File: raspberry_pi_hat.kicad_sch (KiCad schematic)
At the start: 30 parts, among them J1 CONN_JTAG, J3 Conn_01x08, J4 475890001, P1 CONN_02X20, U1 93LC56BT-I_OT, U2 FT232H, Y1 CSTNE12M0G550000R0

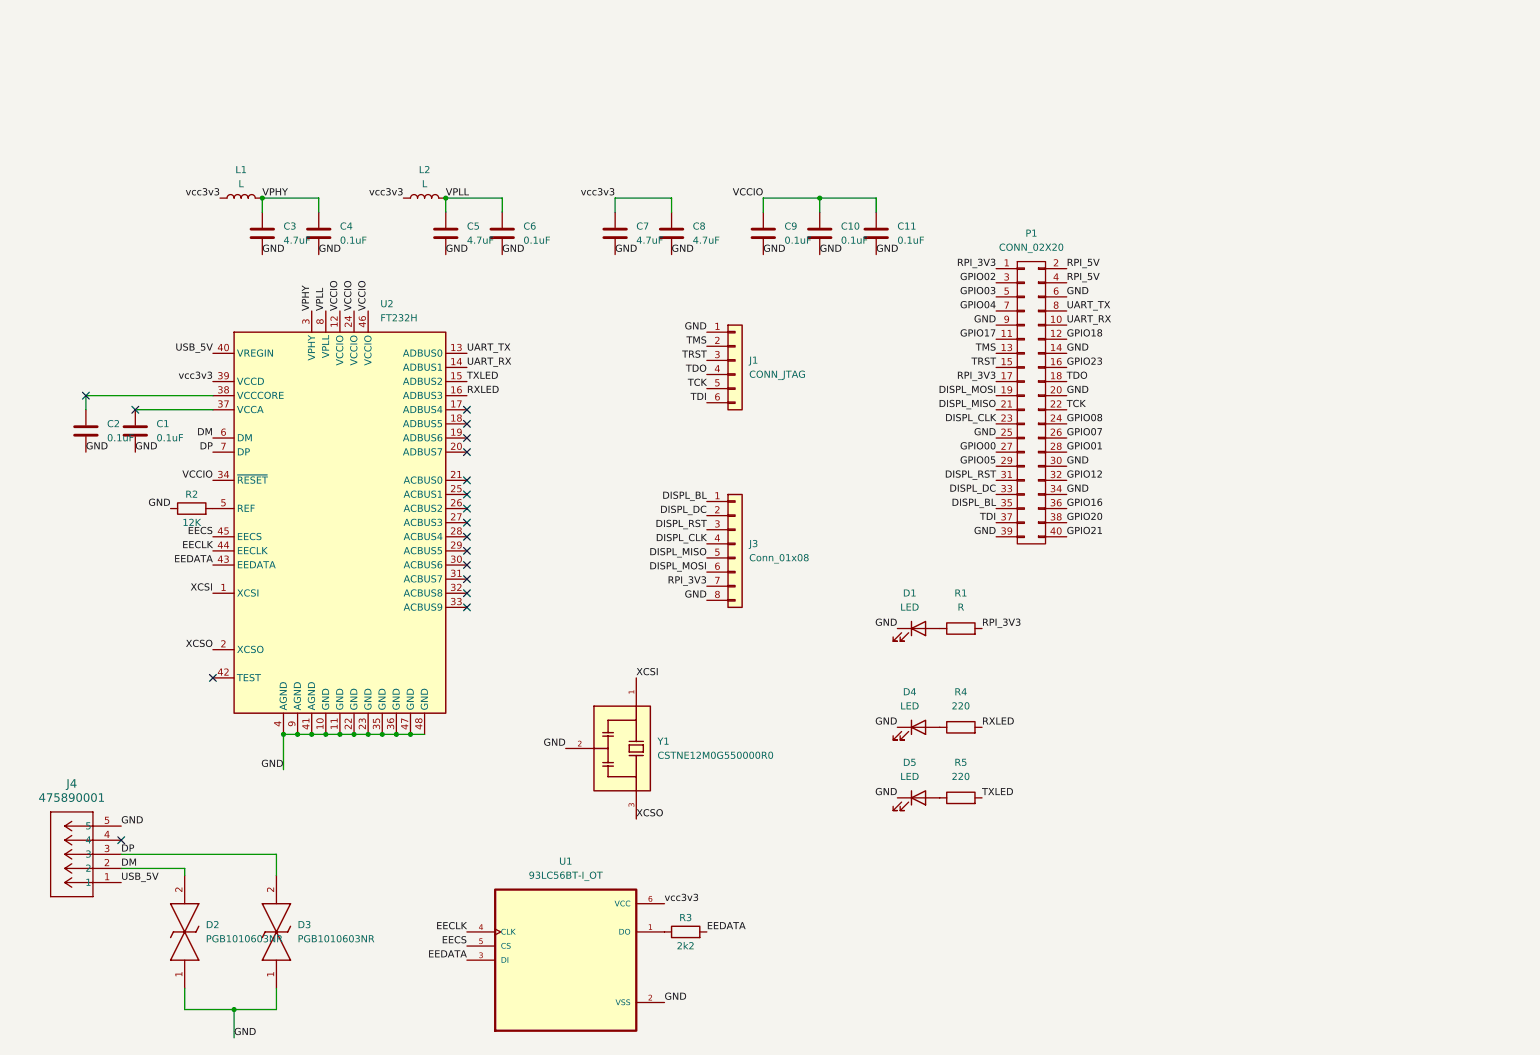
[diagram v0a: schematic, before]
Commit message: progress
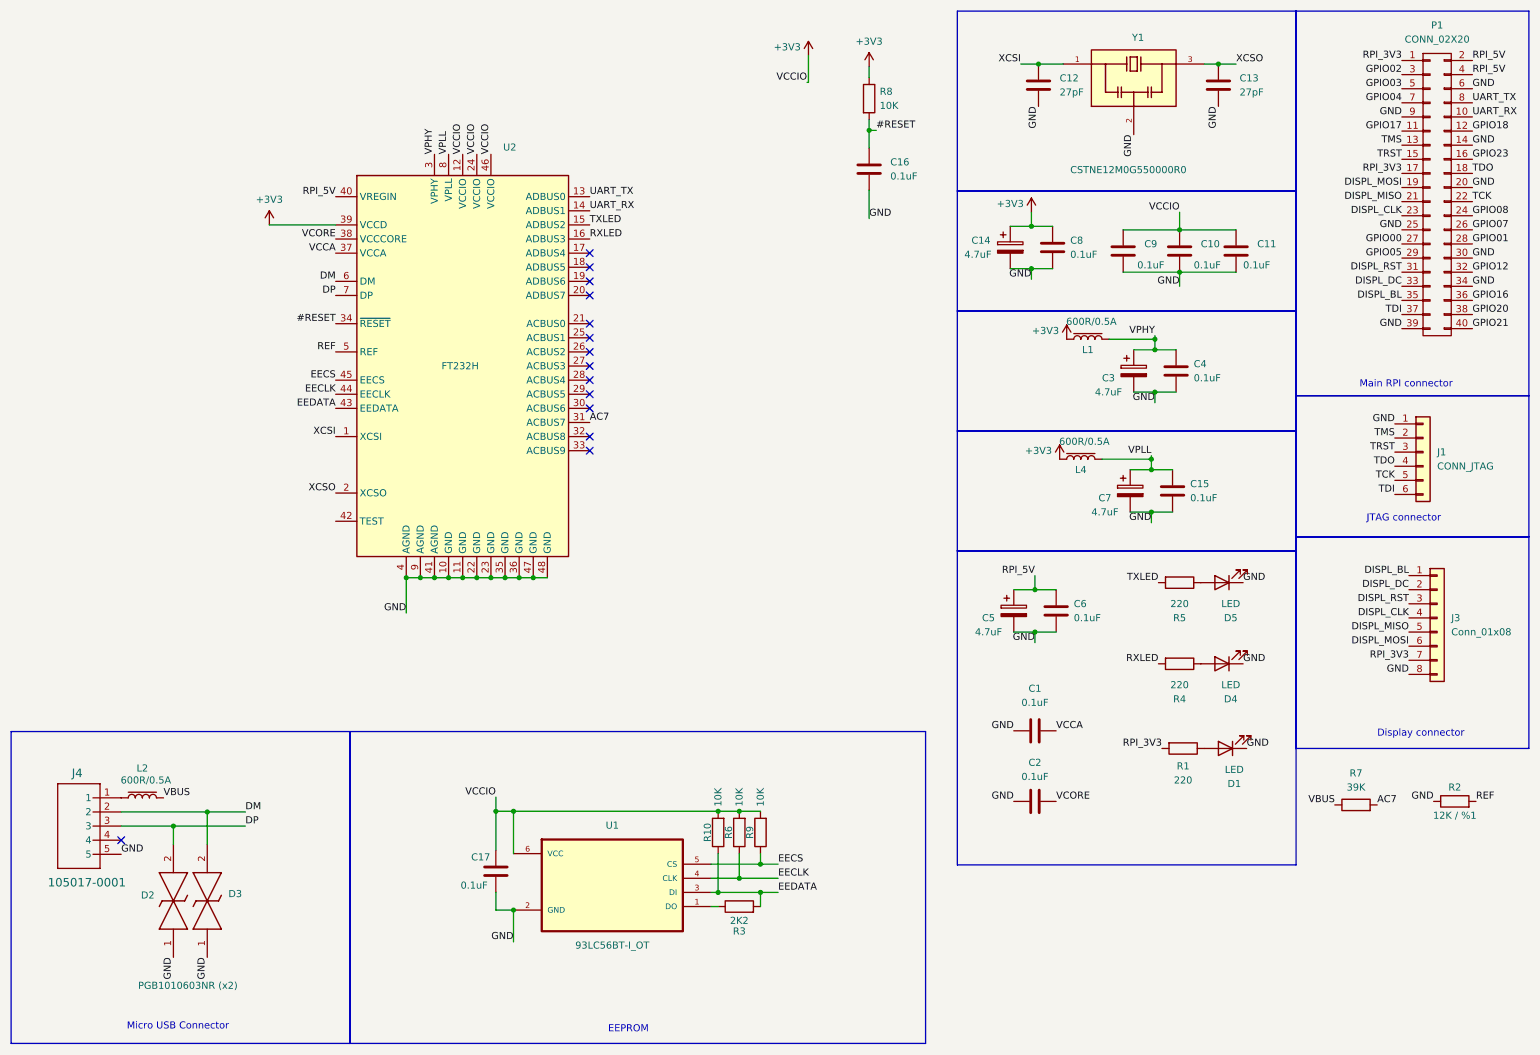
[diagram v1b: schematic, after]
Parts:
- removed C3, C5, C7: 4.7uF, Capacitor_SMD:C_0504_1310Metric_Pad0.83x1.28mm_HandSolder, symbol Device:C
- removed L1, L2: L, Inductor_SMD:L_1008_2520Metric, symbol Device:L
- added C12, C13: 27pF, Capacitor_SMD:C_0201_0603Metric_Pad0.64x0.40mm_HandSolder, symbol Device:C
- added C14, C3, C5, C7: 4.7uF, footprints:CAPPM2014X120N, symbol Device:C_Polarized
- added C15, C16, C17: 0.1uF, Capacitor_SMD:C_0201_0603Metric_Pad0.64x0.40mm_HandSolder, symbol Device:C
- added L1, L2, L4: 600R/0.5A, footprints:BLM21AG102BH1J, symbol Device:L_Iron
- added R10, R6, R8, R9: 10K, Resistor_SMD:R_0201_0603Metric_Pad0.64x0.40mm_HandSolder, symbol Device:R
- added R7: 39K, Resistor_SMD:R_0201_0603Metric_Pad0.64x0.40mm_HandSolder, symbol Device:R
- C1, C10, C11, C2, C4, C6, C9: footprint Capacitor_SMD:C_0504_1310Metric_Pad0.83x1.28mm_HandSolder -> Capacitor_SMD:C_0201_0603Metric_Pad0.64x0.40mm_HandSolder
- C8: value 4.7uF -> 0.1uF; footprint Capacitor_SMD:C_0504_1310Metric_Pad0.83x1.28mm_HandSolder -> Capacitor_SMD:C_0201_0603Metric_Pad0.64x0.40mm_HandSolder
- D2: value PGB1010603NR -> PGB1010603NR (x2)
- J4: value 475890001 -> 105017-0001; Product (none) -> https://www.mouser.fr/ProductDetail/Molex/105017-0001?qs=hl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
- R1: value R -> 220; footprint Resistor_SMD:R_0603_1608Metric -> Resistor_SMD:R_0201_0603Metric_Pad0.64x0.40mm_HandSolder
- R2: value 12K -> 12K / %1; footprint Resistor_SMD:R_0402_1005Metric_Pad0.72x0.64mm_HandSolder -> Resistor_SMD:R_0201_0603Metric_Pad0.64x0.40mm_HandSolder
- R3: value 2k2 -> 2K2; footprint Resistor_SMD:R_0402_1005Metric_Pad0.72x0.64mm_HandSolder -> Resistor_SMD:R_0201_0603Metric_Pad0.64x0.40mm_HandSolder
- R4, R5: footprint Resistor_SMD:R_0603_1608Metric -> Resistor_SMD:R_0201_0603Metric_Pad0.64x0.40mm_HandSolder
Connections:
- net vcc3v3 is gone; now on net +3V3: C8.1, U1.6 (VCC), U2.39 (VCCD)
- net DM: now also D3.2; no longer D2.2
- net DP: now also D2.2; no longer D3.2
- net EECLK: now also R6.1
- net EECS: now also R9.1
- net EEDATA: now also R10.1
- net GND: now also C1.1, C2.1, C12.1, C13.1, C14.2, C15.2, C16.2, C17.2, C3.2, C5.2, C7.2; no longer C1.2, C2.2
- net RPI_5V: now also C6.1, U2.40 (VREGIN), C5.1
- net VPHY: now also C3.1, L1.2
- net VPLL: now also C15.1, C7.1, L4.2; no longer C6.1
- net XCSI: now also C12.2
- net XCSO: now also C13.2
- net REF: now reaches R2.2, U2.5 (REF)
- net VCCA: now reaches U2.37 (VCCA)
- net VCCA: now also C1.2; no longer C1.1
- net AC7: now reaches U2.31 (ACBUS7)
- net AC7: now also R7.2
- net VCORE: now reaches U2.38 (VCCCORE)
- net VCORE: now also C2.2; no longer C2.1
- net USB_5V: no longer names the net of J4.1
- net USB_5V: now also L2.1; no longer U2.40 (VREGIN)
- net VCCIO renamed +3V3
- net +3V3: now also C14.1, C17.1, L1.1, L4.1, R10.2, R6.2, R8.1, R9.2; no longer U2.34 (~{RESET})
- new net #RESET: C16.1, R8.2, U2.34 (~{RESET})
- new net VBUS: L2.2, R7.1
- no-connect marks 18 -> 14
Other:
- note added: "Display connector"
- note added: "EEPROM"
- note added: "JTAG connector"
- note added: "Main RPI connector"
- note added: "Micro USB Connector"
- moved on the sheet: C1, C10, C11, C2, C8, C9, D1, D2, D3, D4, D5, J1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
